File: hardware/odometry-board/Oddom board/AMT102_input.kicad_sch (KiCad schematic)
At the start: 7 parts, among them J4 Conn_01x04, U3 74LVC2G17

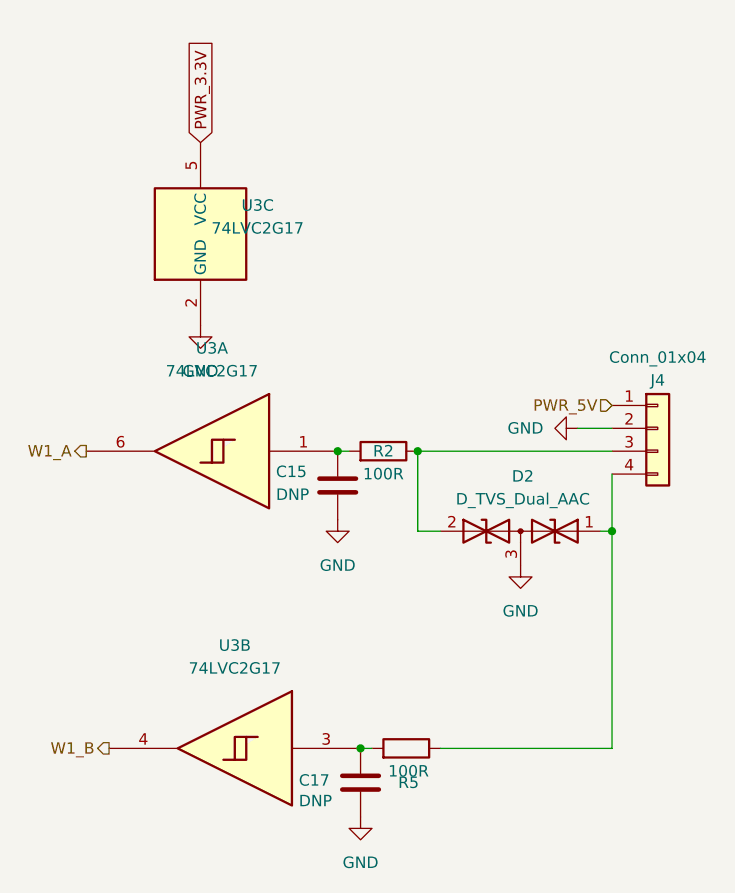
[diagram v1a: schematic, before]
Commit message: WIP: route odometry board RevA
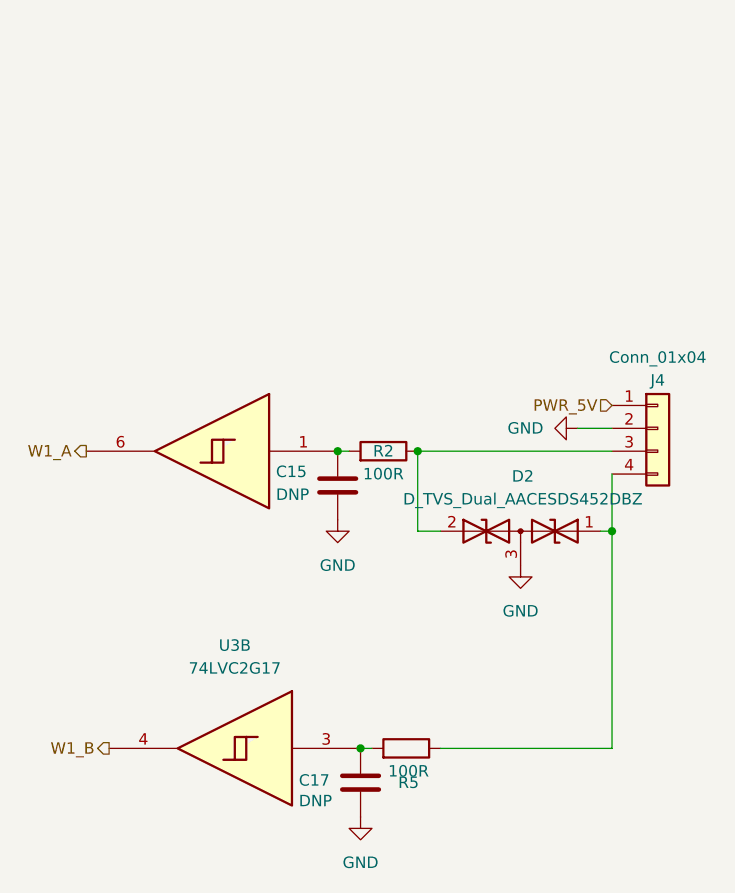
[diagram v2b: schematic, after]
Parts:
- removed unit 3 of U3
- D2: value D_TVS_Dual_AAC -> D_TVS_Dual_AACESDS452DBZ; footprint (none) -> Package_TO_SOT_SMD:SOT-23
- U3: footprint (none) -> Package_TO_SOT_SMD:SOT-23-6
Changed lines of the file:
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@@
-		)
-	)
-	(global_label "PWR_3.3V"
-		(shape input)
-		(at 134.62 35.56 90)
-		(fields_autoplaced yes)
-		(effects
-			(font
-				(size 1.27 1.27)
-			)
-			(justify left)
-		)
-		(property "Intersheetrefs" "${INTERSHEET_REFS}"
-			(at 134.62 35.56 0)
-			(hide yes)
-			(show_name no)
-			(do_not_autoplace no)
-			(effects
-				(font
-					(size 1.27 1.27)
-				)
-				(justify left)
-			)
 		)
 	)
@@
 	(symbol
 		(lib_id "power:GND")
-		(at 134.62 55.88 0)
-		(unit 1)
-		(body_style 1)
-		(exclude_from_sim no)
-		(in_bom yes)
-		(on_board yes)
-		(in_pos_files yes)
-		(dnp no)
-		(fields_autoplaced yes)
-		(property "Reference" "#PWR044"
-			(at 134.62 62.23 0)
-			(hide yes)
-			(show_name no)
-			(do_not_autoplace no)
-			(effects
-				(font
-					(size 1.27 1.27)
-				)
-			)
-		)
-		(property "Value" "GND"
-			(at 134.62 60.96 0)
-			(show_name no)
-			(do_not_autoplace no)
-			(effects
-				(font
-					(size 1.27 1.27)
-				)
-			)
-		)
-		(property "Footprint" ""
-			(at 134.62 55.88 0)
-			(hide yes)
-			(show_name no)
-			(do_not_autoplace no)
-			(effects
-				(font
-					(size 1.27 1.27)
-				)
-			)
-		)
-		(property "Datasheet" ""
-			(at 134.62 55.88 0)
-			(hide yes)
-			(show_name no)
-			(do_not_autoplace no)
-			(effects
-				(font
-					(size 1.27 1.27)
-				)
-			)
-		)
-		(property "Description" "Power symbol creates a global label with name \"GND\" , ground"
-			(at 134.62 55.88 0)
-			(hide yes)
-			(show_name no)
-			(do_not_autoplace no)
-			(effects
-				(font
-					(size 1.27 1.27)
-				)
-			)
-		)
-		(pin "1"
-		)
-		(instances
-			(project "Oddom board"
-				(path "/fb6eb458-0fd8-4f13-9fe8-a6967e1b6388/23269436-26fb-417a-a3a6-ce38dc93169d"
-					(reference "#PWR044")
-					(unit 1)
-				)
-				(path "/fb6eb458-0fd8-4f13-9fe8-a6967e1b6388/6a5e2450-3d09-4f25-8f35-f26d3b9197d2"
-					(reference "#PWR045")
-					(unit 1)
-				)
-				(path "/fb6eb458-0fd8-4f13-9fe8-a6967e1b6388/6b620a29-8bb4-4149-b42a-2d9191ba5545"
-					(reference "#PWR046")
-					(unit 1)
-				)
-			)
-		)
-	)
-	(symbol
-		(lib_id "power:GND")
 		(at 149.86 77.47 0)
 		(mirror y)
@@
 			)
 		)
-		(property "Value" "D_TVS_Dual_AAC"
+		(property "Value" "D_TVS_Dual_AACESDS452DBZ"
 			(at 170.434 75.184 0)
 			(show_name no)
@@
 			)
 		)
-		(property "Footprint" ""
+		(property "Footprint" "Package_TO_SOT_SMD:SOT-23"
 			(at 173.99 78.74 0)
 			(hide yes)
@@
 	)
 	(symbol
-		(lib_id "74xGxx:74LVC2G17")
-		(at 134.62 45.72 0)
-		(unit 3)
-		(body_style 1)
-		(exclude_from_sim no)
-		(in_bom yes)
-		(on_board yes)
-		(in_pos_files yes)
-		(dnp no)
-		(fields_autoplaced yes)
-		(property "Reference" "U3"
-			(at 140.97 42.545 0)
-			(show_name no)
-			(do_not_autoplace no)
-			(effects
-				(font
-					(size 1.27 1.27)
-				)
-			)
-		)
-		(property "Value" "74LVC2G17"
-			(at 140.97 45.085 0)
-			(show_name no)
-			(do_not_autoplace no)
-			(effects
-				(font
-					(size 1.27 1.27)
-				)
-			)
-		)
-		(property "Footprint" ""
-			(at 134.62 45.72 0)
-			(hide yes)
-			(show_name no)
-			(do_not_autoplace no)
-			(effects
-				(font
-					(size 1.27 1.27)
-				)
-			)
-		)
-		(property "Datasheet" "http://www.ti.com/lit/sg/scyt129e/scyt129e.pdf"
-			(at 134.62 45.72 0)
-			(hide yes)
-			(show_name no)
-			(do_not_autoplace no)
-			(effects
-				(font
-					(size 1.27 1.27)
-				)
-			)
-		)
-		(property "Description" "Dual Buffer, Schmitt Triggered, Low-Voltage CMOS"
-			(at 134.62 45.72 0)
-			(hide yes)
-			(show_name no)
-			(do_not_autoplace no)
-			(effects
-				(font
-					(size 1.27 1.27)
-				)
-			)
-		)
-		(pin "1"
-		)
-		(pin "6"
-		)
-		(pin "3"
-		)
-		(pin "4"
-		)
-		(pin "5"
-		)
-		(pin "2"
-		)
-		(instances
-			(project "Oddom board"
-				(path "/fb6eb458-0fd8-4f13-9fe8-a6967e1b6388/23269436-26fb-417a-a3a6-ce38dc93169d"
-					(reference "U3")
-					(unit 3)
-				)
-				(path "/fb6eb458-0fd8-4f13-9fe8-a6967e1b6388/6a5e2450-3d09-4f25-8f35-f26d3b9197d2"
-					(reference "U7")
-					(unit 3)
-				)
-				(path "/fb6eb458-0fd8-4f13-9fe8-a6967e1b6388/6b620a29-8bb4-4149-b42a-2d9191ba5545"
-					(reference "U9")
-					(unit 3)
-				)
-			)
-		)
-	)
-	(symbol
 		(lib_id "Device:C")
 		(at 152.4 106.68 0)
@@
 			)
 		)
-		(property "Footprint" ""
+		(property "Footprint" "Package_TO_SOT_SMD:SOT-23-6"
 			(at 137.16 102.87 0)
 			(hide yes)
@@
 		(property "Reference" "U3"
 			(at 135.89 58.42 0)
+			(hide yes)
 			(show_name no)
 			(do_not_autoplace no)
@@
 		(property "Value" "74LVC2G17"
 			(at 135.89 60.96 0)
-			(show_name no)
-			(do_not_autoplace no)
-			(effects
-				(font
-					(size 1.27 1.27)
-				)
-			)
-		)
-		(property "Footprint" ""
+			(hide yes)
+			(show_name no)
+			(do_not_autoplace no)
+			(effects
+				(font
+					(size 1.27 1.27)
+				)
+			)
+		)
+		(property "Footprint" "Package_TO_SOT_SMD:SOT-23-6"
 			(at 134.62 69.85 0)
 			(hide yes)
